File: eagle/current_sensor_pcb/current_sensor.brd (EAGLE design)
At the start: 160 x 100 mm, 1 part, among them M1 ARDUINO-NANO-LONG

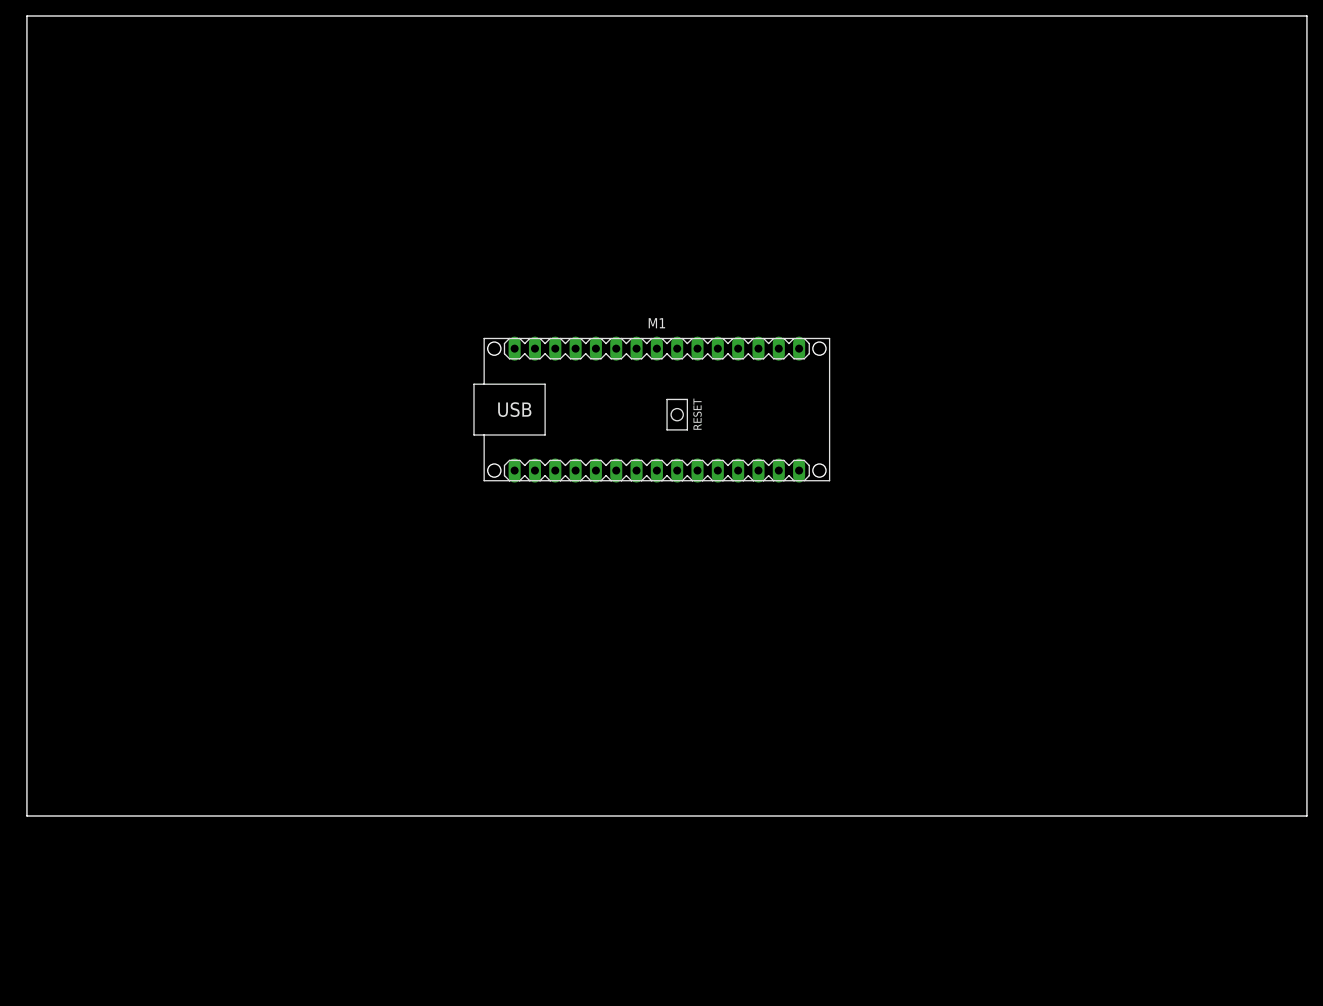
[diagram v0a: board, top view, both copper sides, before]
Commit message: pcb design ready
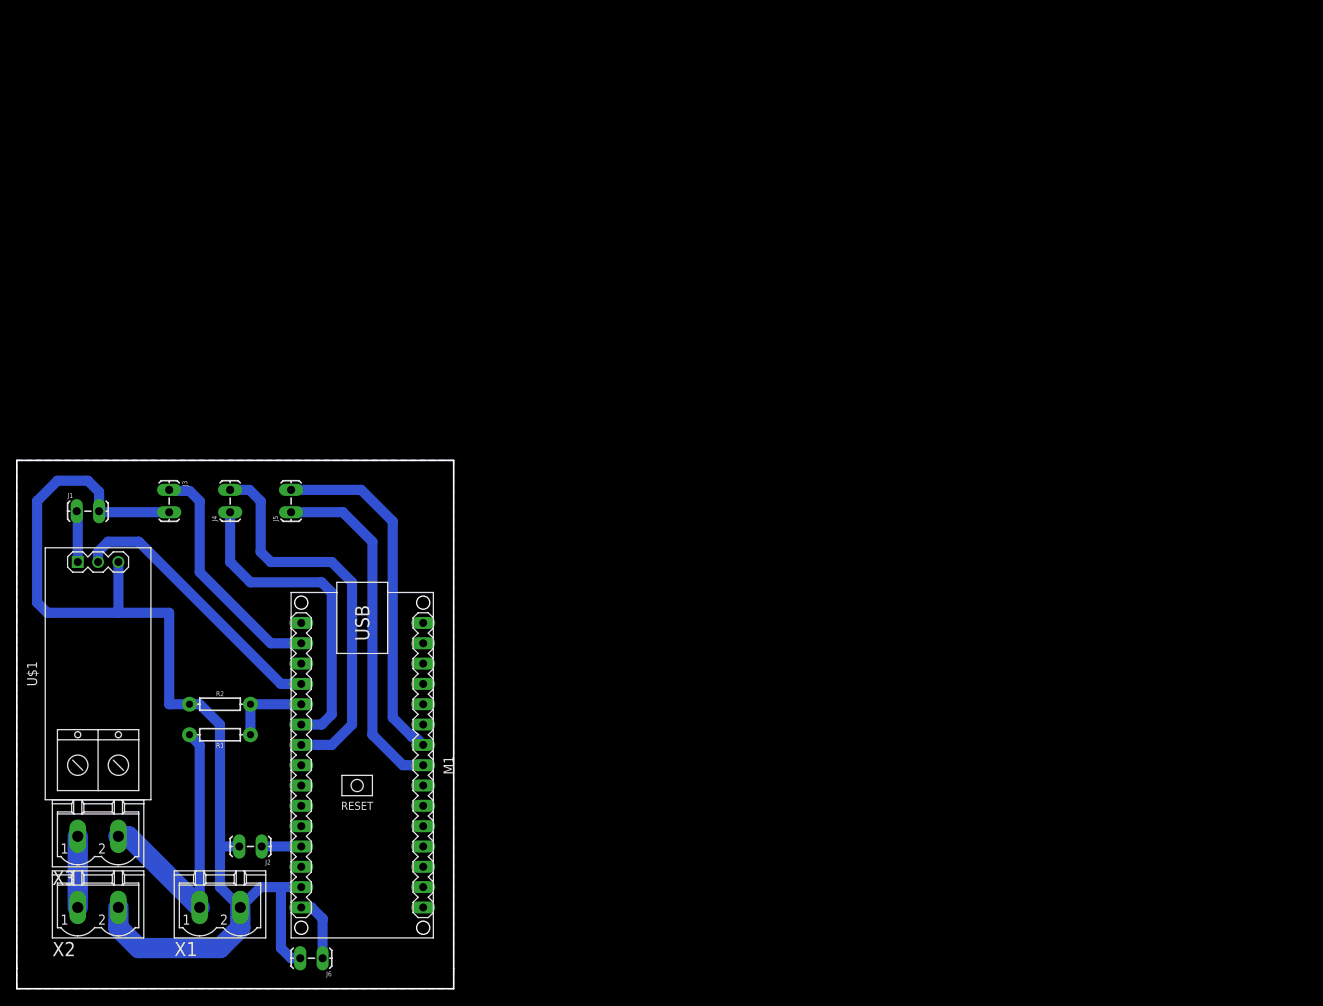
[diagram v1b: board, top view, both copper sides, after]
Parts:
- added J1, J2, J3, J4, J5, J6: (no value), SparkFun-Connectors:1X02_LOCK_LONGPADS
- added R1, R2: (no value), SparkFun-Resistors:AXIAL-0.3
- added U$1: CURRENT-SENSOR-ACS712, diy-modules:CURRENT-SENSOR-ACS712
- added X1, X2, X3: MST2V, con-phoenix-508:MSTBV2
- moved M1 57.7 mm to (41.9, 6.35), turned to 270 degrees
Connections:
- removed net GND.2: M1.J2.2
- new net A2: J4.1, M1.J2.10
- new net A3: J4.2, M1.J2.9
- new net D5: J5.1, M1.J1.8
- new net D6: J5.2, M1.J1.9
- new net GND: J1.2, J2.2, J3.2, J6.2, M1.J2.2, R2.P$1, U$1.3, X1.2, X2.2
- new net N$1: M1.J2.12, U$1.2
- new net N$2: R1.P$2, X1.1, X3.2
- new net N$3: J1.1, U$1.1
- new net N$5: M1.J2.11, R1.P$1, R2.P$2
- new net N$6: X2.1, X3.1
- net 3V3: now also J3.1
- net 5V: now also J2.1
- net VIN: now also J6.1
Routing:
- net GND: track 0.00 -> 143.5 mm
- net A3: track 0.00 -> 48.9 mm
- net D6: track 0.00 -> 44.1 mm
- net D5: track 0.00 -> 43.7 mm
- net A2: track 0.00 -> 40.3 mm
- net N$2: track 0.00 -> 36.0 mm
- net N$1: track 0.00 -> 34.6 mm
- net 3V3: track 0.00 -> 29.8 mm
- net N$5: track 0.00 -> 10.2 mm
- net N$6: track 0.00 -> 8.89 mm
- net VIN: track 0.00 -> 8.20 mm
- net N$3: track 0.00 -> 6.40 mm
- net 5V: track 0.00 -> 4.95 mm
- added copper zone on layer 1, net GND
- added copper zone on layer 16, net GND
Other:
- board size 160 x 100 mm -> 54.6 x 66 mm
